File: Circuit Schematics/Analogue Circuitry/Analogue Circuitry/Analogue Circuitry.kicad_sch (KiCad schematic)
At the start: 37 parts

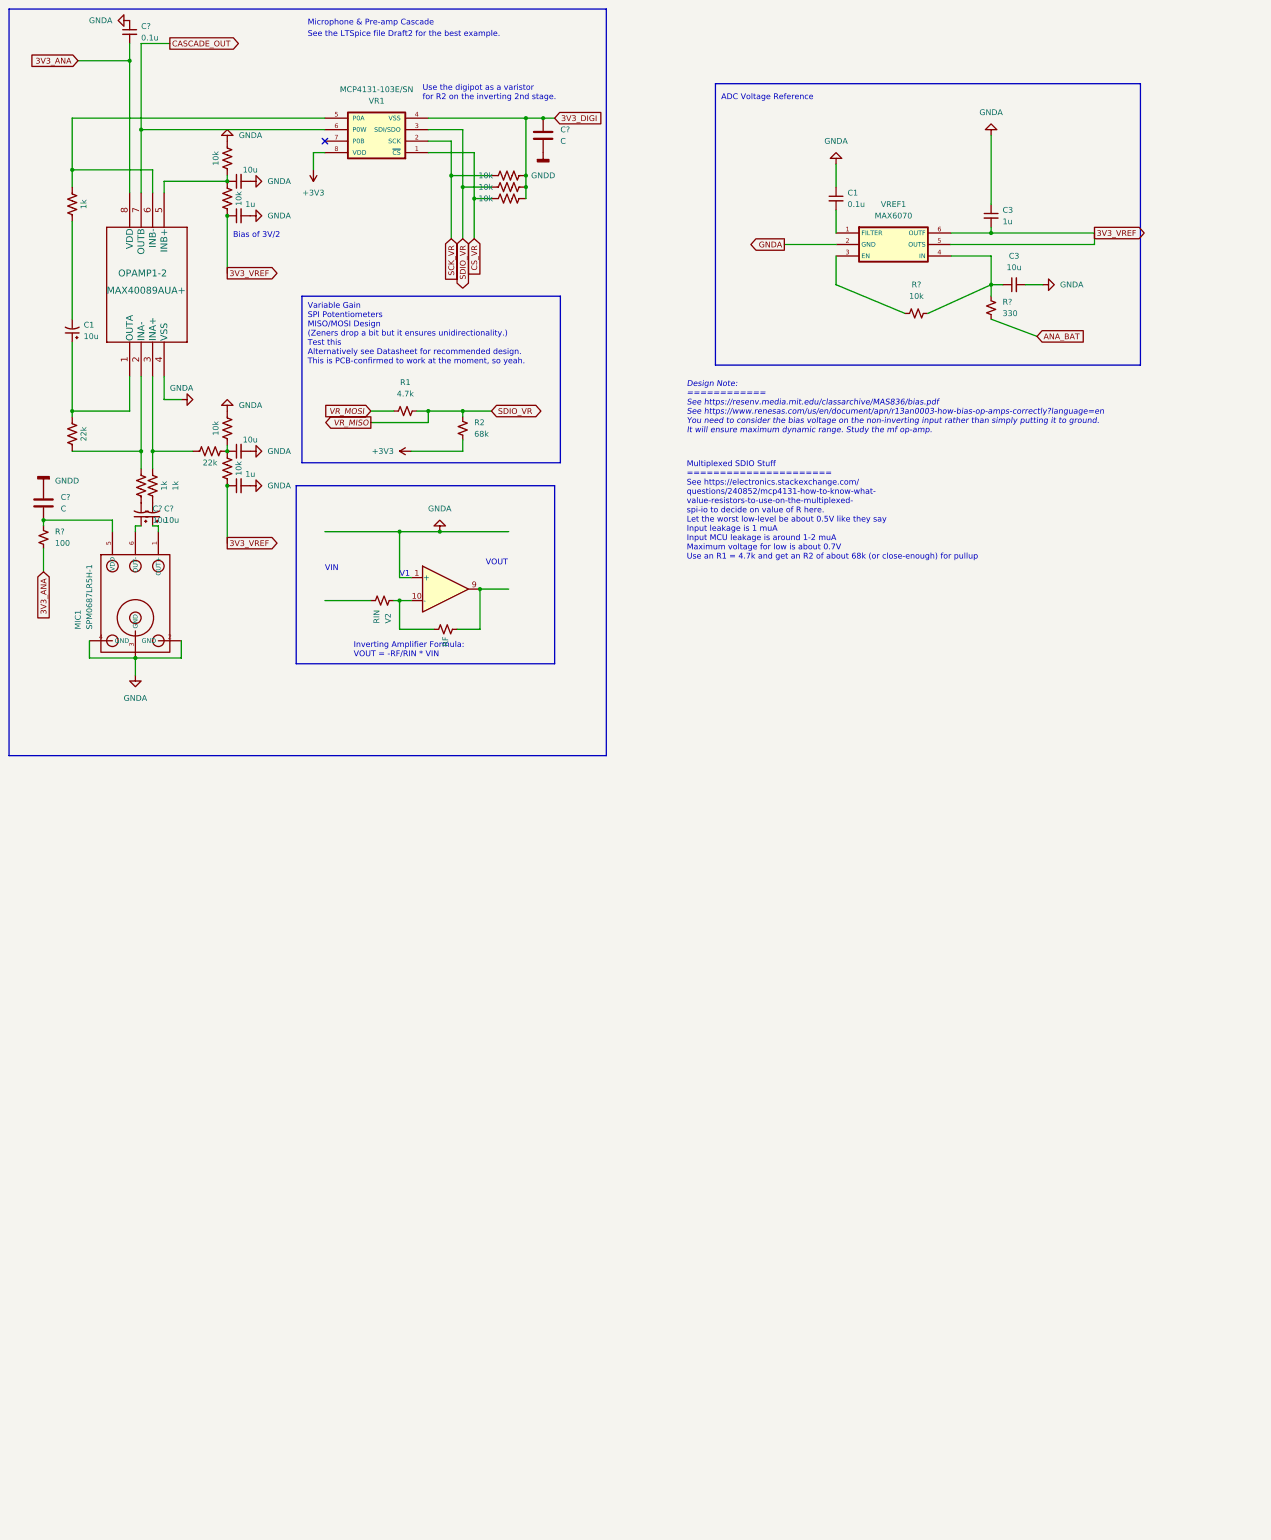
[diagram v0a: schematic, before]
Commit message: Bunch of changes
and I'm a lazy mofo who doesn't want to version control my directory and so yeah
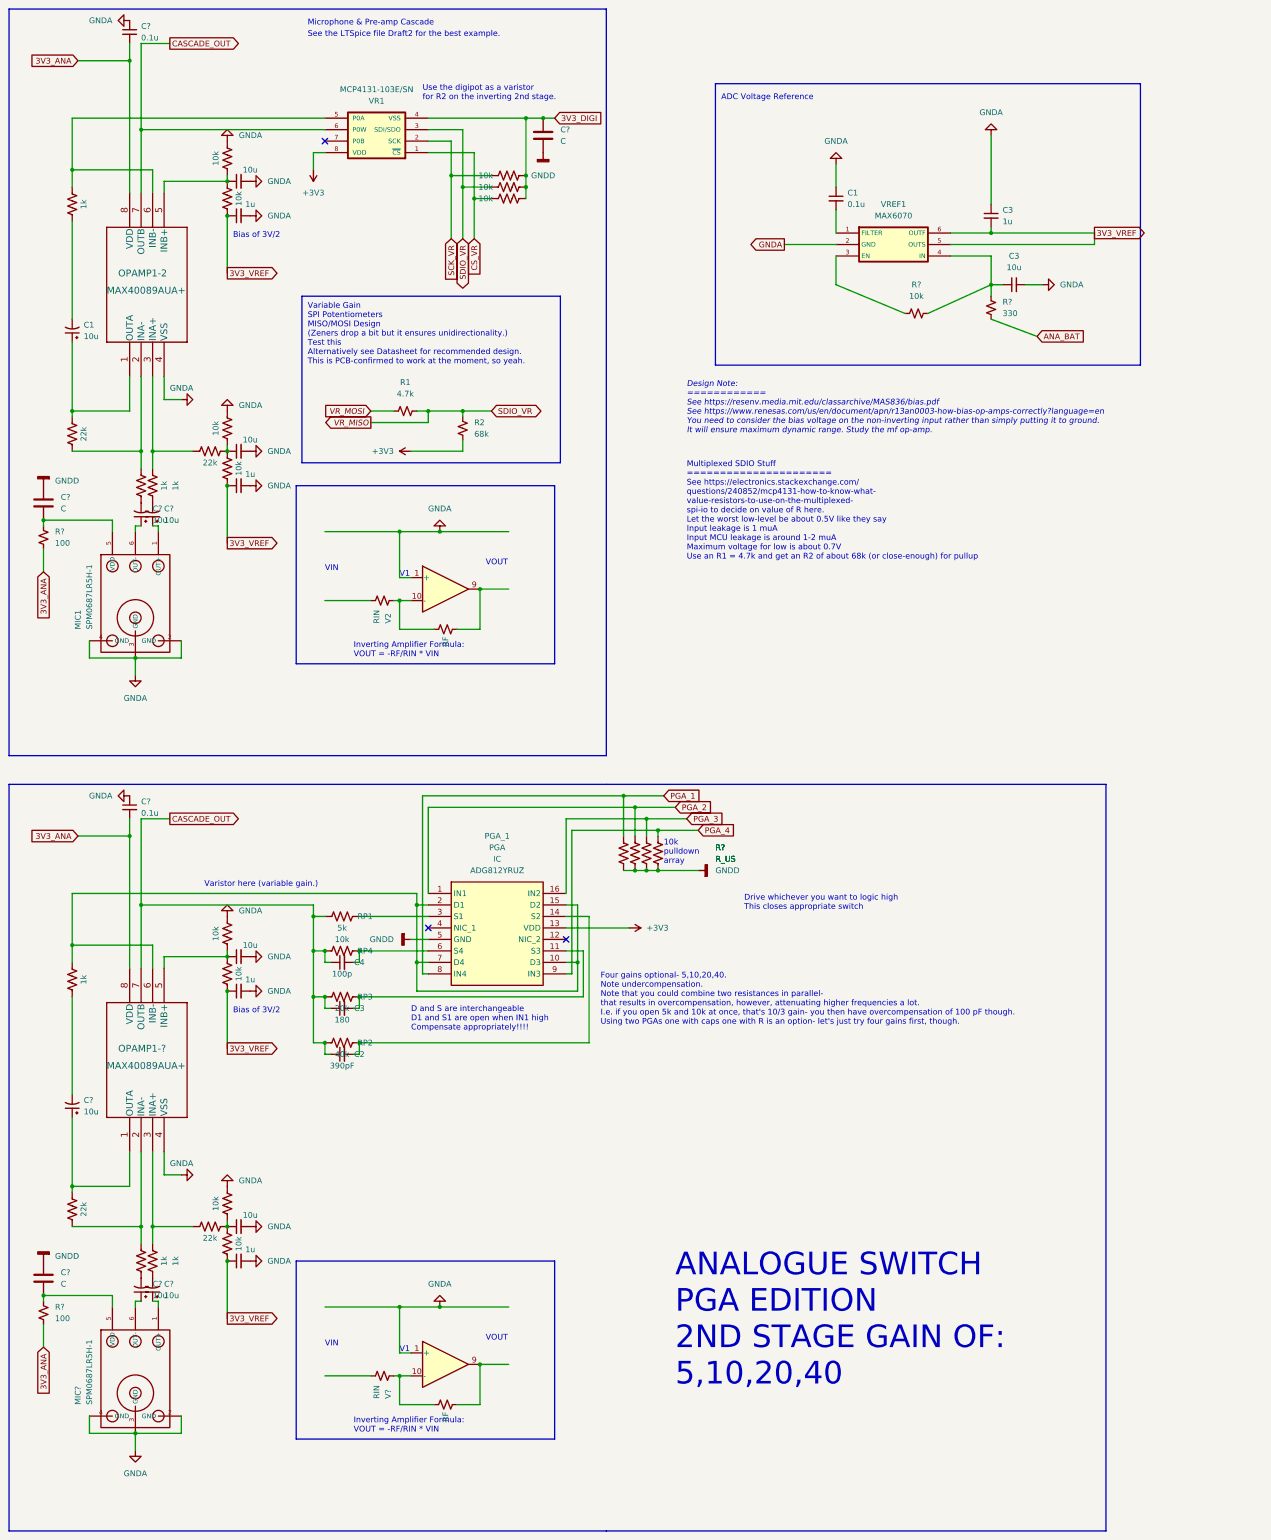
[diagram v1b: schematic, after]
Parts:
- added C2: 390pF, symbol Device:C_Small
- added C3: 180, symbol Device:C_Small
- added C4: 100p, symbol Device:C_Small
- added C?: 0.1u, symbol Device:C_Small
- added C? (x2): 10u, symbol Device:C_Small
- added C? (x3): 10u, symbol Device:C_Polarized_Small_US
- added C?: C, symbol Device:C
- added C? (x2): 1u, symbol Device:C_Small
- added MIC?: SPM0687LR5H-1, symbol SPM0687LR5H-1:SPM0687LR5H-1
- added O?: OPA, Package_SON:Texas_S-PVSON-N10, symbol Amplifier_Audio:OPA1622
- added OPAMP1-?: MAX40089AUA+, 21-0036K_MXM, symbol MAX40089AUA+:MAX40089AUA+
- added PGA_1: PGA, symbol ADG812YRUZ:ADG812YRUZ
- added R? (x3): 1k, symbol Device:R_US
- added R? (x4), RP4: 10k, symbol Device:R_US
- added R? (x4): R_US, symbol Device:R_US
- added R? (x2): 22k, symbol Device:R_US
- added R?: 100, symbol Device:R_Small_US
- added RP1: 5k, symbol Device:R_US
- added RP2: 40k, symbol Device:R_US
- added RP3: 20k, symbol Device:R_US
- added V?: RIN, symbol Device:R_Small_US
- added V?: RF, symbol Device:R_Small_US
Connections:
- net +3V3: now also PGA_1.13 (VDD)
- net 3V3_ANA: now also C?.2, OPAMP1-?.8 (VDD), R?.1
- net 3V3_VREF: now also C?.1, C?.1, R?.1, R?.1
- net CASCADE_OUT: now also C2.1, C3.1, C4.1, OPAMP1-?.7 (OUTB), RP1.1, RP2.1, RP3.1, RP4.1
- net GNDA: now also C?.1, C?.2, C?.2, C?.2, C?.2, MIC?.2 (GND), MIC?.3 (GND), MIC?.4 (GND), O?.1 (+), OPAMP1-?.4 (VSS), R?.2, R?.2
- net GNDD: now also C?.1, PGA_1.5 (GND), R?.2, R?.2, R?.2, R?.2
- new net: O?.10 (-), V?.1, V?.2
- new net: O?.9, V?.2
- new net: C3.2, PGA_1.11 (S3), RP3.2
- new net: C?.1, OPAMP1-?.5 (INB+), R?.1, R?.2
- new net: C?.1, OPAMP1-?.1 (OUTA), R?.2
- new net: C?.2, R?.1 (x3)
- new net: C2.2, PGA_1.14 (S2), RP2.2
- new net: OPAMP1-?.3 (INA+), R?.2, R?.2
- new net: PGA_1.3 (S1), RP1.2
- new net: C?.2, MIC?.5 (VDD), R?.2
- new net: C?.1, MIC?.1 (OUT+)
- new net: C?.1, MIC?.6 (OUT-)
- new net: OPAMP1-?.2 (INA-), R?.1, R?.2
- new net: C4.2, PGA_1.6 (S4), RP4.2
- new net: OPAMP1-?.6 (INB-), PGA_1.10 (D3), PGA_1.15 (D2), PGA_1.2 (D1), PGA_1.7 (D4), R?.2
- new net: C?.1, R?.1, R?.1, R?.2
- new net PGA_1: PGA_1.8 (IN4), R?.1
- new net PGA_2: PGA_1.1 (IN1), R?.1
- new net PGA_3: PGA_1.16 (IN2), R?.1
- new net PGA_4: PGA_1.9 (IN3), R?.1
- no-connect marks 1 -> 3
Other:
- note added: "10k pulldown array"
- note added: "ANALOGUE SWITCH PGA EDITION 2ND STAGE GAIN OF: 5,10,20,40"
- note added: "D and S are interchangeable D1 and S1 are open when IN1 high Compensate appropriately!!!!"
- note added: "Drive whichever you want to logic high This closes appropriate switch"
- note added: "Four gains optional- 5,10,20,40. Note undercompensation. Note that you could combine two resistances in parallel- that results in overcompensation, however, attenuating higher frequencies a lot. I.e. if you open 5k and 10k at once, that's 10/3 gain- you then have overcompensation of 100 pF though. Using two PGAs one with caps one with R is an option- let's just try four gains first, though."
- note added: "Varistor here (variable gain.)"
